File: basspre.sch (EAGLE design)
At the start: 6 parts, among them IC1 LF351D

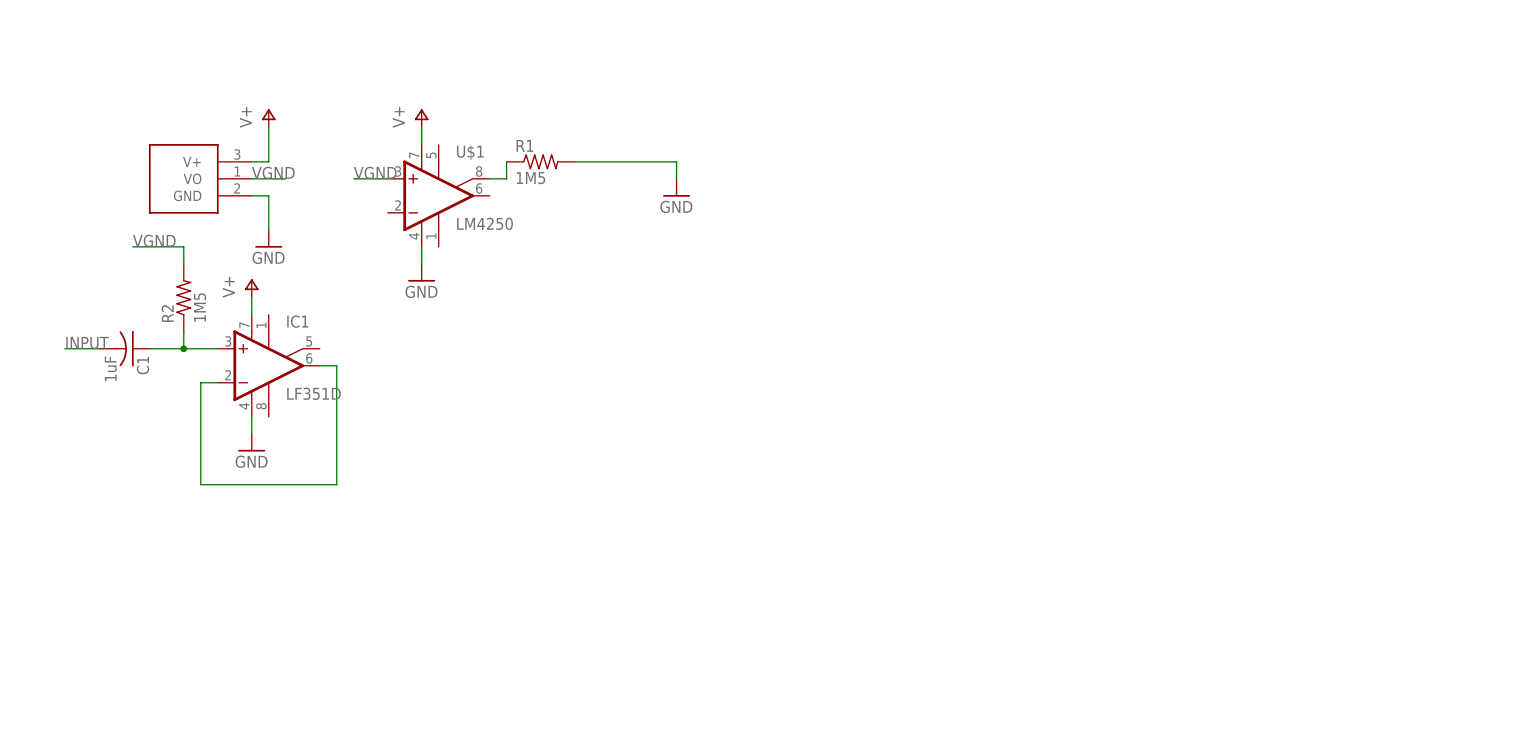
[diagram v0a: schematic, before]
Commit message: initial layout
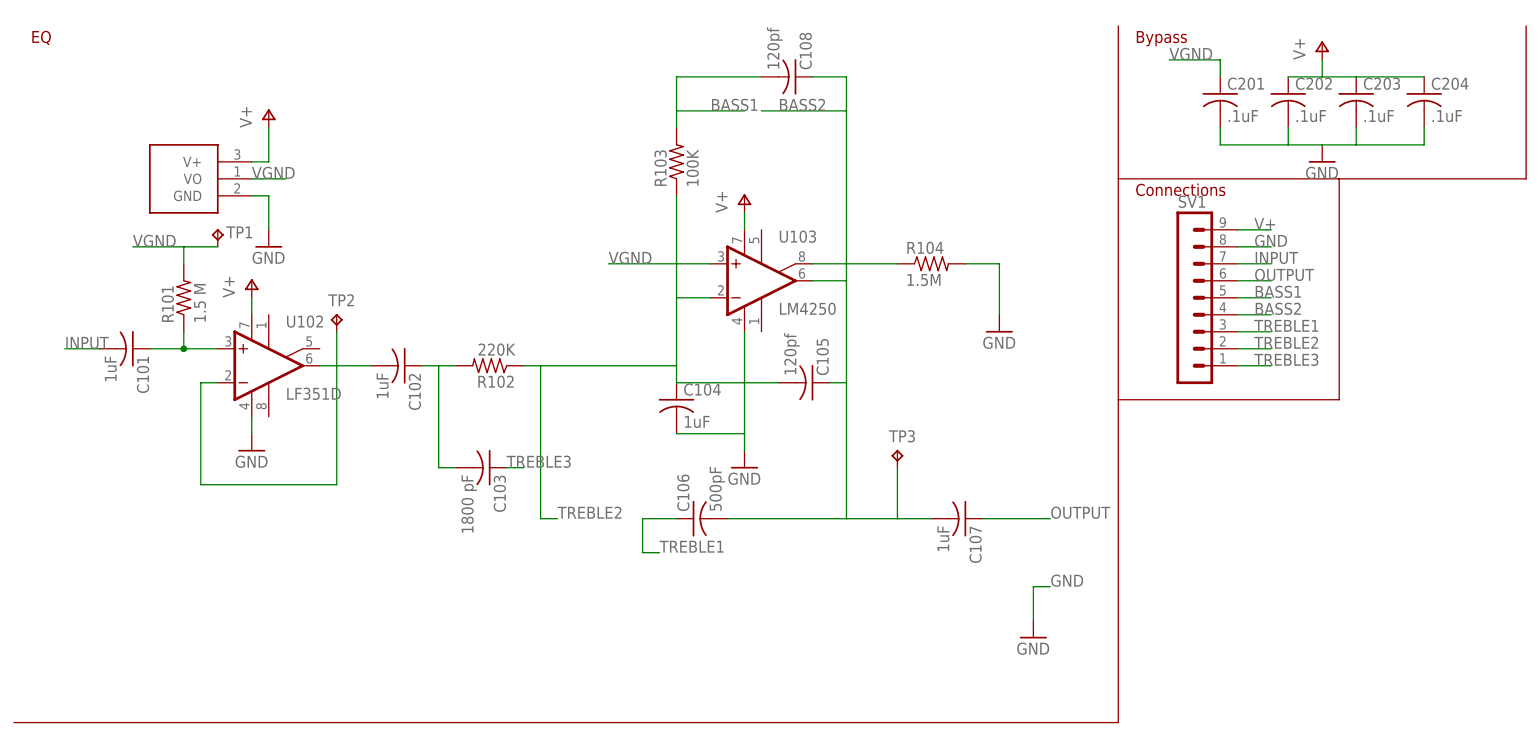
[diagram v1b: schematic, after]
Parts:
- removed R1: 1M5, resistor:R-US_R0603
- removed U$1: LM4250, russell_random:LM4250
- added C102, C104, C107: 1uF, resistor:C-USC0603
- added C103: 1800 pF, resistor:C-USC0603
- added C105, C108: 120pf, resistor:C-USC0603
- added C106: 500pF, resistor:C-USC0603
- added C201, C202, C203, C204: .1uF, resistor:C-USC0603
- added R102: 220K, resistor:R-US_R0603
- added R103: 100K, resistor:R-US_R0603
- added R104: 1.5M, resistor:R-US_R0603
- added SV1: (no value), con-lstb:MA09-1
- added TP1, TP2, TP3: TPPAD1-13, testpad:TPPAD1-13
- added U103: LM4250, russell_random:LM4250
- R101: value 1M5 -> 1.5 M
- renumbered C1 to C101, IC1 to U102, R2 to R101, U$2 to U101
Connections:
- new net BASS1: C108.2, R103.2, SV1.5
- new net BASS2: C105.1, C106.2, C107.2, C108.1, SV1.4, TP3.TP, U103.OUT
- new net N$1: C102.1, C103.2, R102.2
- new net OUTPUT: C107.1, SV1.6
- new net TREBLE1: C106.1, SV1.3
- new net TREBLE2: C104.1, C105.2, R102.1, R103.1, SV1.2, U103.-IN
- new net TREBLE3: C103.1, SV1.1
- net GND: now also C104.2, C201.2, C202.2, C203.2, C204.2, R104.2, SV1.8, U103.V-; no longer R1.2, U$1.V-
- net INPUT: now also SV1.7
- net N$2: now also R104.1, U103.CURRENT; no longer R1.1, U$1.CURRENT
- net N$3: now also C102.2, TP2.TP
- net V+: now also C202.1, C203.1, C204.1, SV1.9, U103.V+; no longer U$1.V+
- net VGND: now also C201.1, TP1.TP, U103.+IN; no longer U$1.+IN
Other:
- note added: "Bypass"
- note added: "Connections"
- note added: "EQ"
